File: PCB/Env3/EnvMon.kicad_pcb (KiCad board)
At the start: 2 copper layers, 70 x 70 mm, 46 parts, among them J1 LCD, J2 DC, J3 TEMP, J4 LCD, J5 Reset, J6 USB-C-Socket-H, J7 TC2030-USB-NL-DS, U1 ESP32-S3-MINI-1, U2 SCD41, U3 MD8942, U4 MCP9808_MSOP, U5 GZP6816D, U8 VEML6040

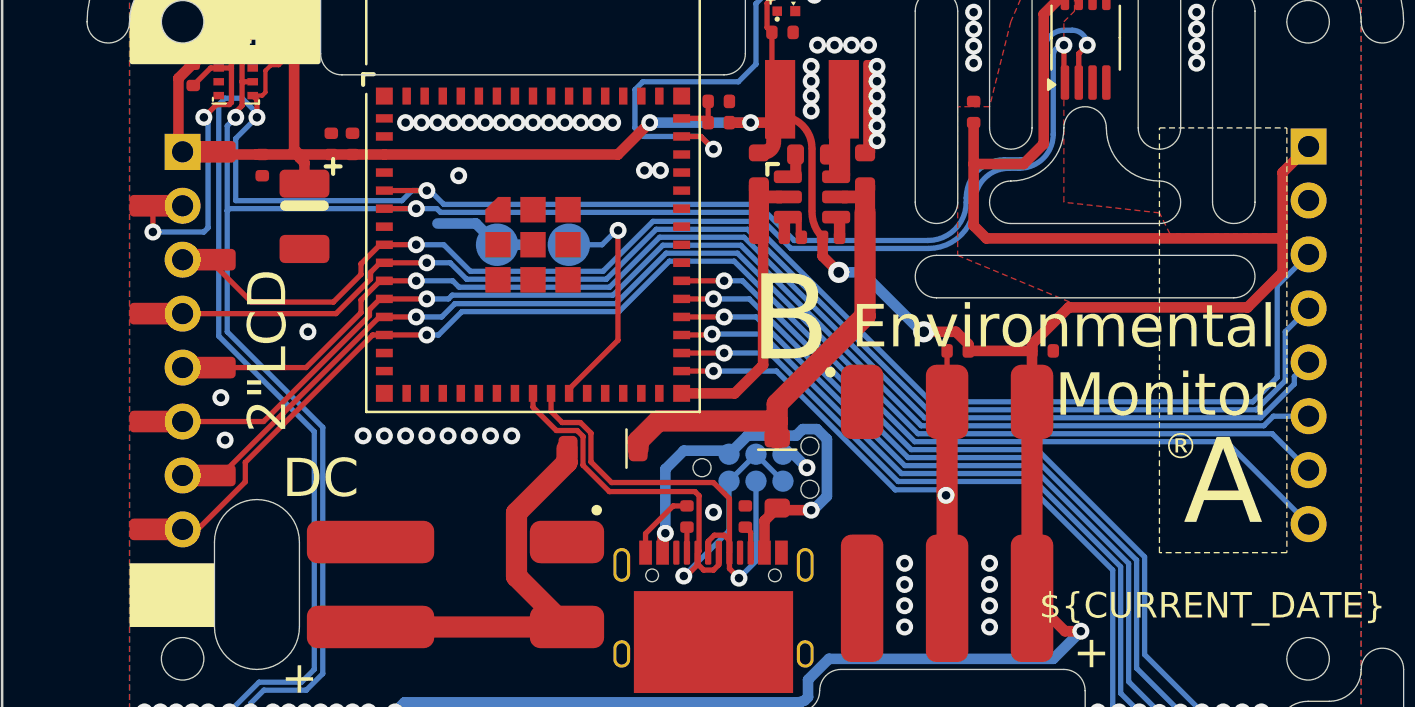
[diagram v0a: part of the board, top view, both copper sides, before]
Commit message: Library update
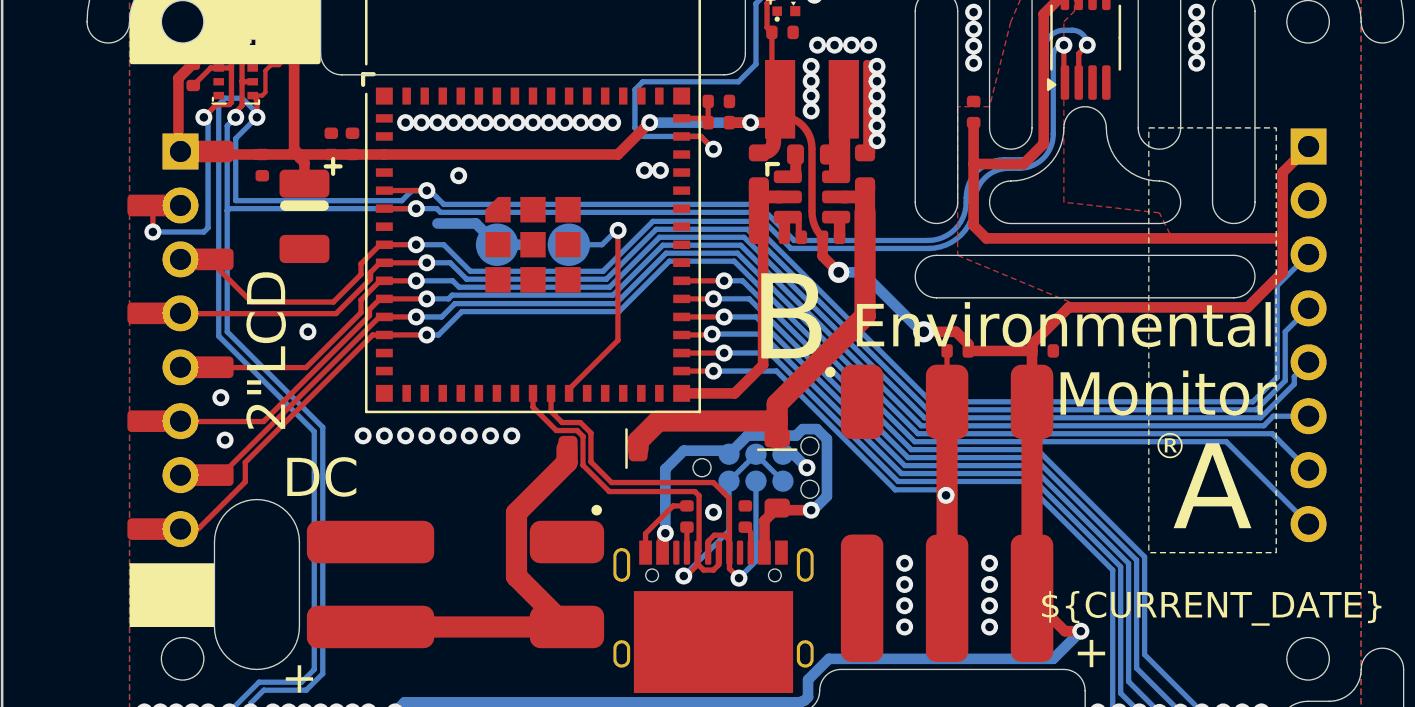
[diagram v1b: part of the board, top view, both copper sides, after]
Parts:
- J1: footprint RevK:PinSocket_1x08_P2.54mm_Vertical_SMD -> RevK:LCD2
- moved J1 0.10 mm to (73.4, 83.6)
